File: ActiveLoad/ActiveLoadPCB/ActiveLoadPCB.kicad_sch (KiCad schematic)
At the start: 56 parts, among them J1 Conn_01x03_Pin, J2 Conn_01x03_Pin, J3 Screw_Terminal_01x02, J4 Screw_Terminal_01x02, J5 Conn_01x03_Pin, J6 Conn_01x03_Pin, J7 LOAD+, J8 LOAD-, Q1 2N2222A, Q10 2N2222A, Q11 TIP142, Q2 2N2222A, Q3 TIP142, Q4 2N2222A, Q5 TIP142, Q6 2N2222A, Q7 TIP142, Q8 2N2222A, Q9 TIP142, U1 LM358

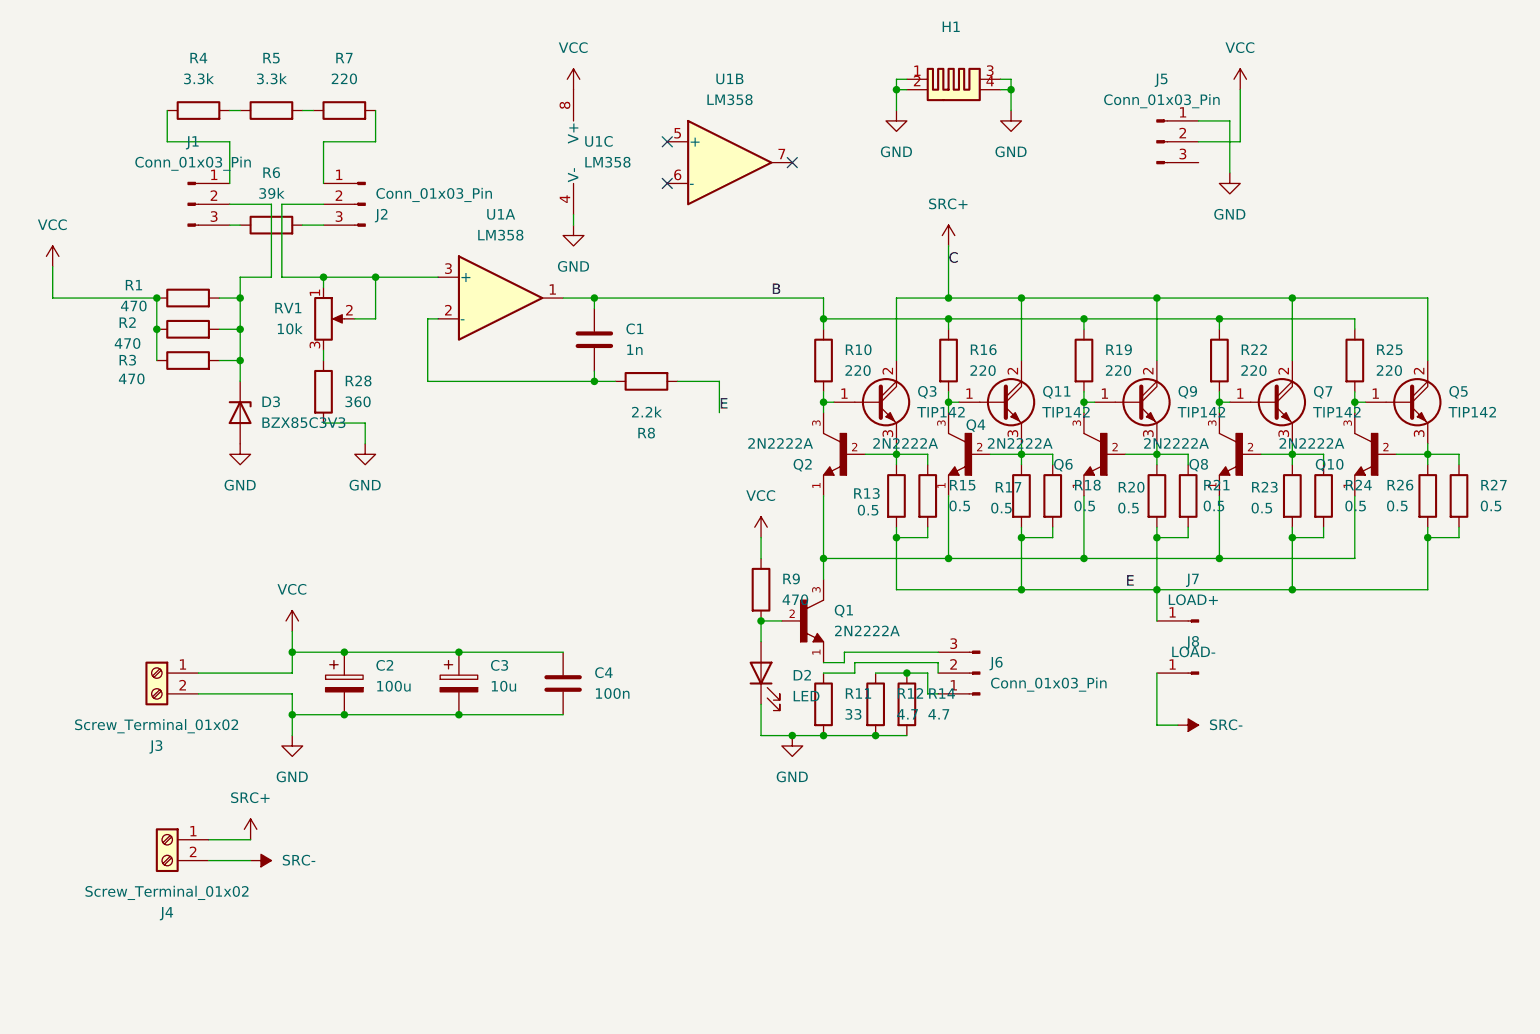
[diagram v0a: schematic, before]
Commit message: Active load PCB second version
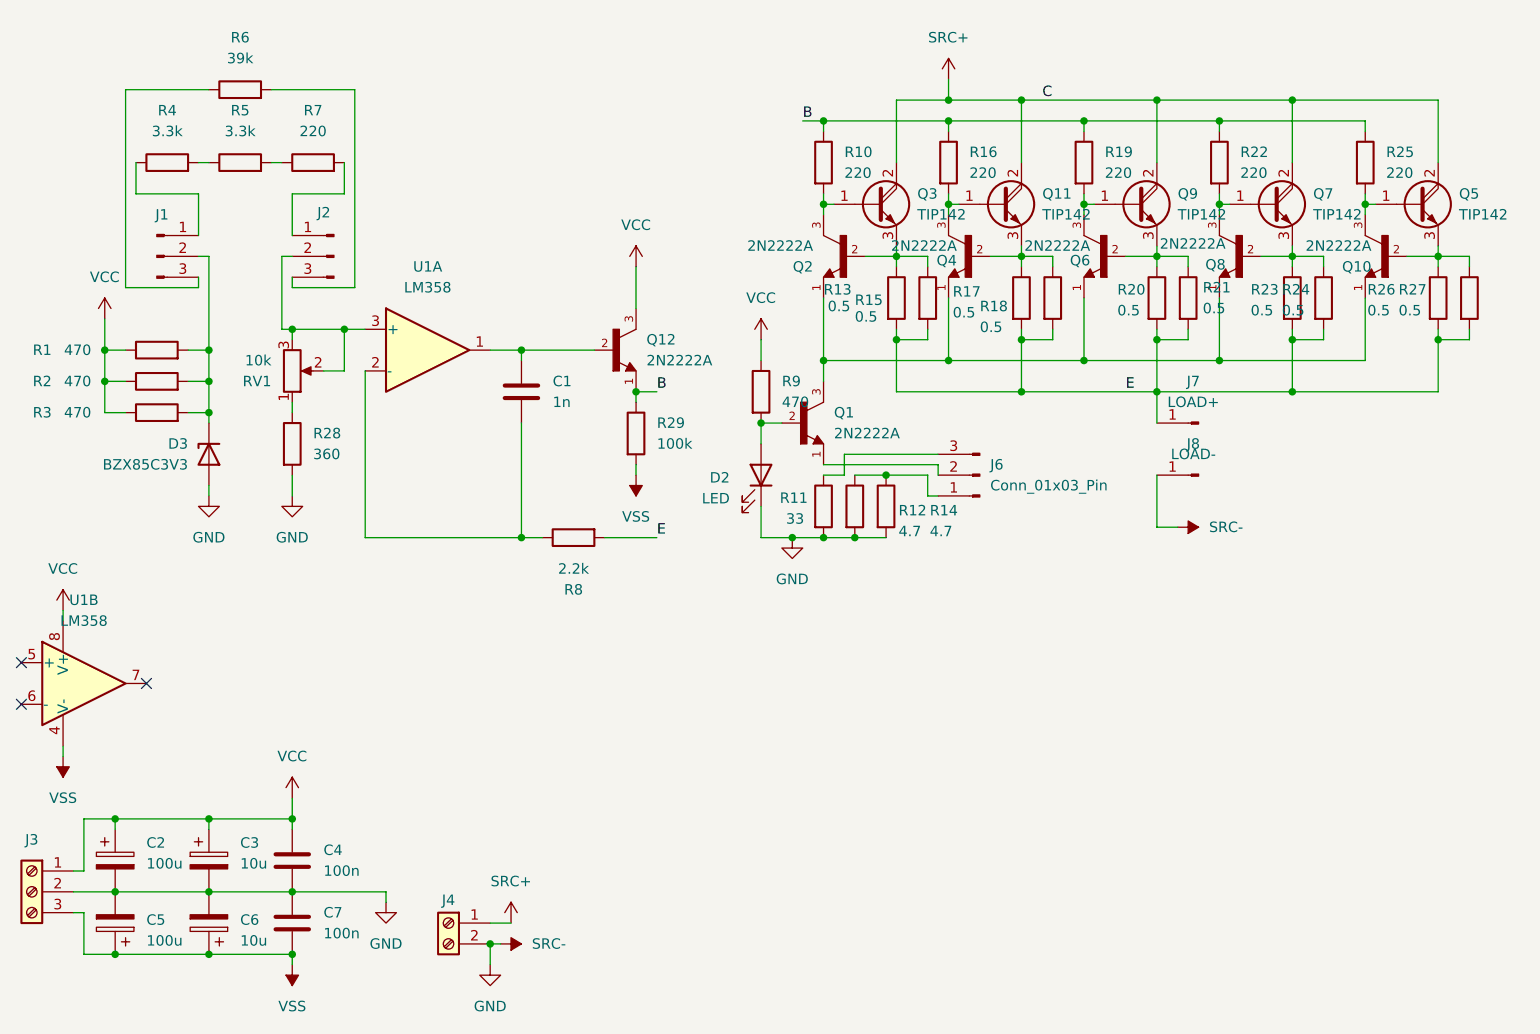
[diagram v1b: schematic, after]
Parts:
- removed H1: ~, Kicad_TitoSync_Footprints:LGA775_Heatsink, symbol KiCad_TitoSync_Symbols:LGA775_Heatsink
- removed J3: Screw_Terminal_01x02, TerminalBlock_4Ucon:TerminalBlock_4Ucon_1x02_P3.50mm_Horizontal, symbol Connector:Screw_Terminal_01x02
- removed J5: Conn_01x03_Pin, Connector_PinHeader_2.00mm:PinHeader_1x03_P2.00mm_Vertical, symbol Connector:Conn_01x03_Pin
- added C5: 100u, Capacitor_THT:CP_Radial_D5.0mm_P2.50mm, symbol Device:C_Polarized
- added C6: 10u, Capacitor_THT:CP_Radial_D5.0mm_P2.50mm, symbol Device:C_Polarized
- added C7: 100n, Capacitor_THT:C_Disc_D5.0mm_W2.5mm_P2.50mm, symbol Device:C
- added J3: Screw_Terminal_01x03, TerminalBlock_MetzConnect:TerminalBlock_MetzConnect_Type055_RT01503HDWU_1x03_P5.00mm_Horizontal, symbol Connector:Screw_Terminal_01x03
- added Q12: 2N2222A, Package_TO_SOT_THT:TO-92L_Inline_Wide, symbol 2N2222A:2N2222A
- added R29: 100k, Resistor_THT:R_Axial_DIN0207_L6.3mm_D2.5mm_P7.62mm_Horizontal, symbol Device:R
- C2, C3: footprint Capacitor_THT:CP_Radial_D5.0mm_P2.00mm -> Capacitor_THT:CP_Radial_D5.0mm_P2.50mm
- J4: footprint TerminalBlock_4Ucon:TerminalBlock_4Ucon_1x02_P3.50mm_Horizontal -> TerminalBlock_MetzConnect:TerminalBlock_MetzConnect_Type055_RT01502HDWU_1x02_P5.00mm_Horizontal
- Q1, Q10, Q2, Q4, Q6, Q8: footprint Package_TO_SOT_THT:TO-92_Inline -> Package_TO_SOT_THT:TO-92L_Inline_Wide
- Q11, Q3, Q5, Q7, Q9: footprint Package_TO_SOT_THT:TO-247-3_Horizontal_TabUp -> Package_TO_SOT_THT:TO-247-3_Vertical
- RV1: footprint Potentiometer_THT:Potentiometer_Alps_RK09Y11_Single_Horizontal -> Kicad_TitoSync_Footprints:Potentiometer
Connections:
- net SRC- is gone; now on net GND: J4.2 (Pin_2), J8.1 (Pin_1)
- net B: now also Q12.1, R29.1; no longer C1.1, U1.1
- net GND: now also C5.2, C6.2, C7.1, J3.2 (Pin_2); no longer U1.4 (V-)
- net VCC: now also J3.1 (Pin_1), Q12.3
- net at Q1.1: now also J6.2 (Pin_2); no longer J6.3 (Pin_3)
- net at J2.2 (Pin_2), RV1.2, U1.3 (+): now also RV1.3; no longer RV1.1
- net at R28.1: now also RV1.1; no longer RV1.3
- net at R11.1: now also J6.3 (Pin_3); no longer J6.2 (Pin_2)
- new net: C1.1, Q12.2, U1.1
- new net VSS: C5.1, C6.1, C7.2, J3.3 (Pin_3), R29.2, U1.4 (V-)
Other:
- moved on the sheet: C1, C2, C3, C4, D2, D3, J1, J2, J4, J6, J7, J8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
